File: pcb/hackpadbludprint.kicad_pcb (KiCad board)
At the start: 2 copper layers, 88.6 x 98 mm, 12 parts, among them SW1 SW_Push, SW2 SW_Push, SW3 SW_Push, SW4 SW_Push, SW5 RotaryEncoder_Switch, U1 MOUDLE-SEEEDUINO-XIAO, U2 ER_OLEDM0.91_1x-I2C

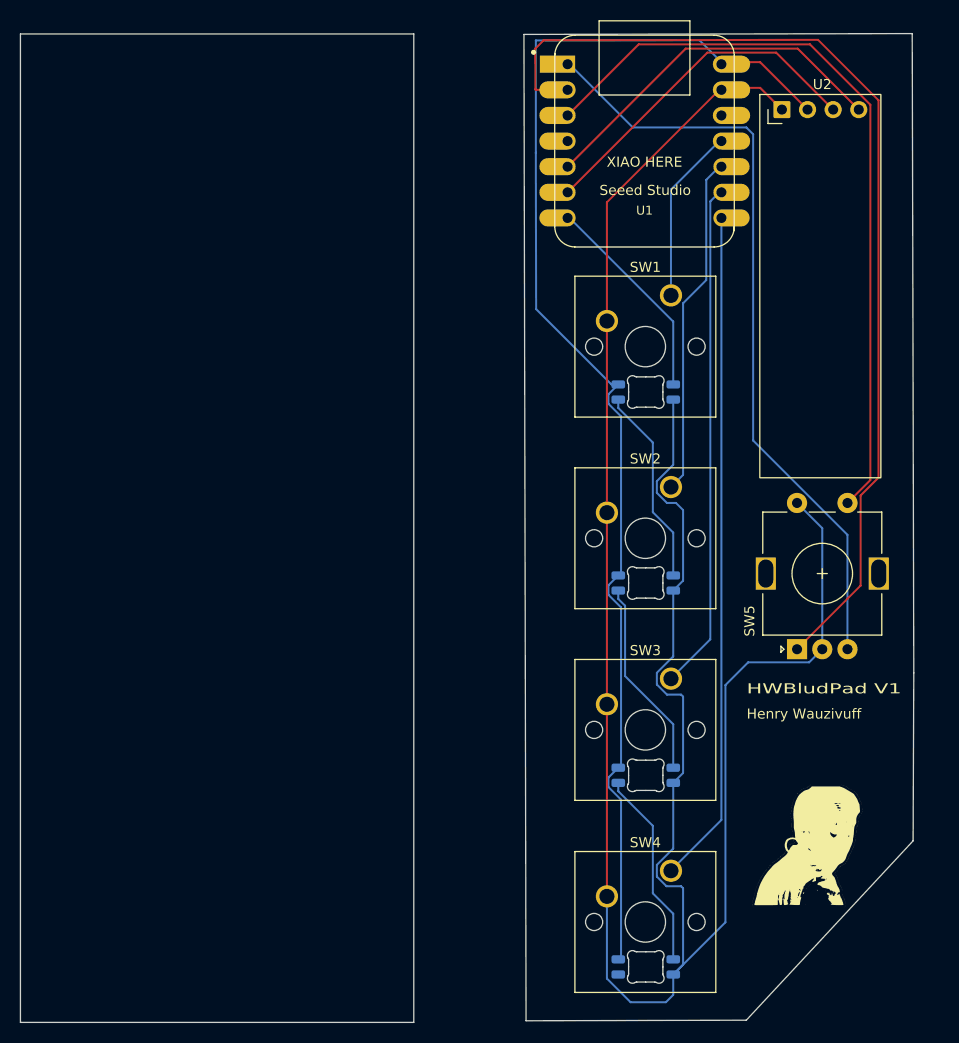
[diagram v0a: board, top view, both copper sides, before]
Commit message: FRIDGEE
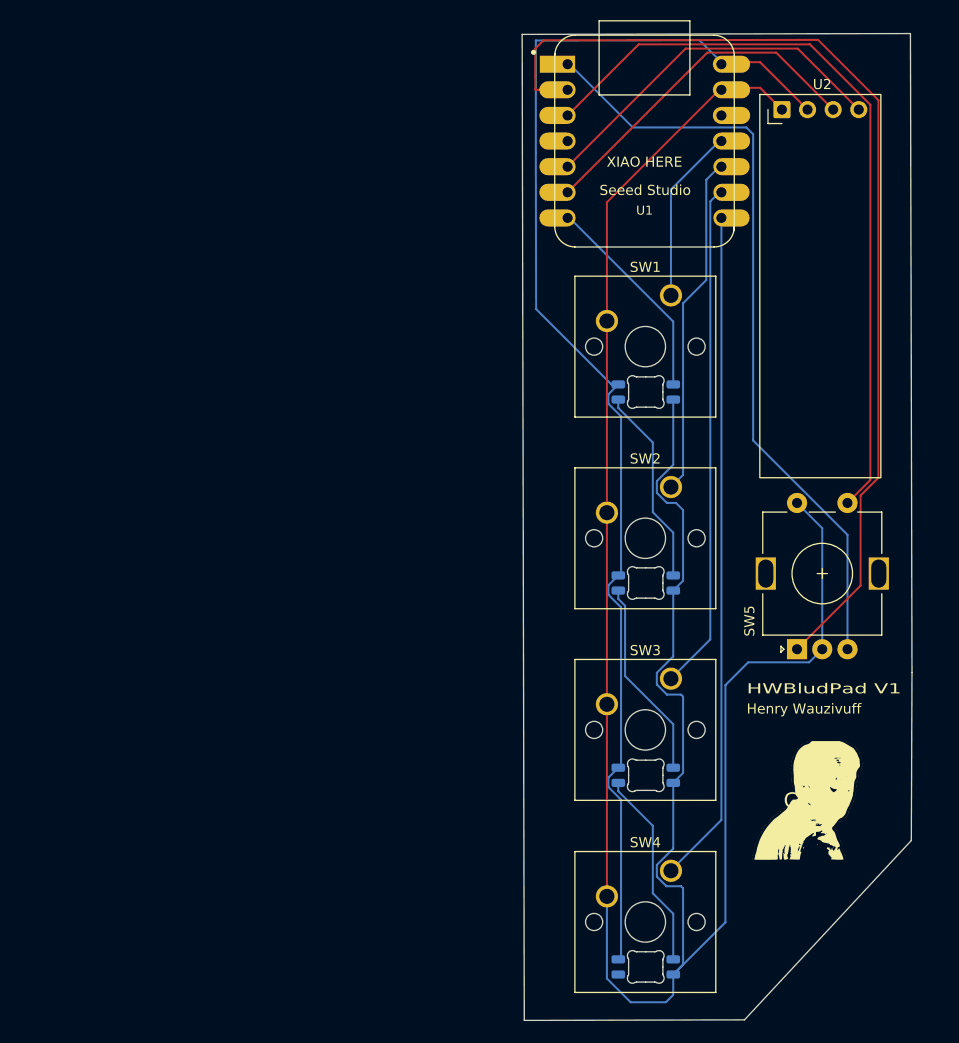
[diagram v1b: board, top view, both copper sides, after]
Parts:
- moved G*** 4.50 mm to (166.5, 126.0)
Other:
- board size 88.6 x 98 mm -> 38.7 x 97.8 mm
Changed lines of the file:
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@@
 	(footprint "projftprints:lawrence_starin"
 		(layer "F.Cu")
-		(at 166.5 130.5)
+		(at 166.5 126)
 		(property "Reference" "G***"
 			(at 0 0 0)
@@
 	(gr_poly
 		(pts
-			(xy 176.919651 49.962542) (xy 138.423379 50.044625) (xy 138.631897 147.83824) (xy 160.466412 147.783309)
-			(xy 177.006951 130) (xy 177.074049 113.341597)
+			(xy 176.742818 49.95897) (xy 138.246536 50.041054) (xy 138.454986 147.802685) (xy 160.289501 147.747754)
+			(xy 176.83004 129.964445) (xy 176.897138 113.306042)
 		)
 		(stroke
@@
 		(layer "Edge.Cuts")
 	)
-	(gr_rect
-		(start 88.5 50)
-		(end 127.5 148)
-		(stroke
-			(width 0.05)
-			(type solid)
-		)
-		(fill no)
-		(layer "Edge.Cuts")
-	)
 	(gr_text "Henry Wauzivuff"
-		(at 160.5 118 0)
+		(at 160.5 117.5 0)
 		(layer "F.SilkS")
 		(effects
@@
 	)
 	(segment
-		(start 167.581533 50.581533)
-		(end 140.363117 50.636883)
+		(start 171.8 104.7)
+		(end 171.8 95.765685)
 		(width 0.2)
 		(layer "F.Cu")
@@
 	)
 	(segment
-		(start 173.57 56.57)
-		(end 167.581533 50.581533)
+		(start 140.359501 50.640499)
+		(end 139.546952 51.453048)
 		(width 0.2)
 		(layer "F.Cu")
@@
 	)
 	(segment
-		(start 165.5 111)
-		(end 171.8 104.7)
+		(start 167.582453 50.582453)
+		(end 140.359501 50.640499)
 		(width 0.2)
 		(layer "F.Cu")
@@
 	)
 	(segment
-		(start 173.57 93.995685)
-		(end 173.57 56.57)
+		(start 173.57 56.57)
+		(end 167.582453 50.582453)
 		(width 0.2)
 		(layer "F.Cu")
@@
 	)
 	(segment
-		(start 140.363117 50.636883)
-		(end 139.546952 51.453048)
+		(start 165.5 111)
+		(end 171.8 104.7)
 		(width 0.2)
 		(layer "F.Cu")
@@
 	)
 	(segment
-		(start 171.8 95.765685)
-		(end 173.57 93.995685)
+		(start 139.595293 55.54)
+		(end 142.75 55.54)
 		(width 0.2)
 		(layer "F.Cu")
@@
 	)
 	(segment
-		(start 139.595293 55.54)
-		(end 142.75 55.54)
+		(start 139.555181 55.499888)
+		(end 139.595293 55.54)
 		(width 0.2)
 		(layer "F.Cu")
@@
 	)
 	(segment
-		(start 171.8 104.7)
-		(end 171.8 95.765685)
+		(start 142.59 55.5)
+		(end 141 55.5)
 		(width 0.2)
 		(layer "F.Cu")
@@
 	)
 	(segment
-		(start 142.59 55.5)
-		(end 141 55.5)
+		(start 173.57 93.995685)
+		(end 173.57 56.57)
 		(width 0.2)
 		(layer "F.Cu")
@@
 	)
 	(segment
-		(start 139.555181 55.499888)
-		(end 139.595293 55.54)
+		(start 171.8 95.765685)
+		(end 173.57 93.995685)
 		(width 0.2)
 		(layer "F.Cu")
